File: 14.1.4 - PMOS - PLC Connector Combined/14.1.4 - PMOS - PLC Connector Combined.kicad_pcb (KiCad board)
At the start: 2 copper layers, 61.5 x 67.8 mm, 110 parts, among them J201 Conn_01x01_PAD, J202 Conn_01x01_PAD, J203 Conn_01x01_PAD, J204 Conn_01x01_PAD, J205 Conn_01x01_PAD, J206 Conn_01x01_PAD, J207 Conn_01x01_PAD, J208 Conn_01x01_PAD, J209 Conn_01x01_PAD, J210 Conn_01x01_PAD, J211 Conn_01x01_PAD, J212 Conn_01x01_PAD, J213 Conn_01x01_PAD, J214 Conn_01x01_PAD, J215 Conn_01x01_PAD, J216 Conn_01x01_PAD, J217 Conn_01x01_PAD, J218 Conn_01x01_PAD, J219 Conn_01x01_PAD, J220 Conn_01x01_PAD, J221 DB128L-5.08-2P-BK-S, J222 DB128L-5.08-2P-BK-S, J223 DB128L-5.08-2P-BK-S, J224 DB128L-5.08-2P-BK-S, J225 DB128L-5.08-2P-BK-S, J226 B04B-XASK-1, J301 Conn_01x01_PAD, J302 Conn_01x01_PAD, J303 Conn_01x01_PAD, J304 Conn_01x01_PAD, J305 Conn_01x01_PAD, J306 Conn_01x01_PAD, J307 Conn_01x01_PAD, J308 Conn_01x01_PAD, J309 Conn_01x01_PAD, J310 Conn_01x01_PAD, J311 Conn_01x01_PAD, J312 Conn_01x01_PAD, J313 Conn_01x01_PAD, J314 Conn_01x01_PAD, J315 Conn_01x01_PAD, J316 Conn_01x01_PAD, J317 DB128L-5.08-2P-BK-S, J318 DB128L-5.08-3P-BK-S, J319 DB128L-5.08-2P-BK-S, J320 DB128L-5.08-2P-BK-S, J321 B04B-XASK-1, Q1 2N7002, Q2 2N7002, Q3 2N7002, Q4 2N7002, U1 DMP6023LE-13, U2 DMP6023LE-13, U3 DMP6023LE-13, U4 DMP6023LE-13

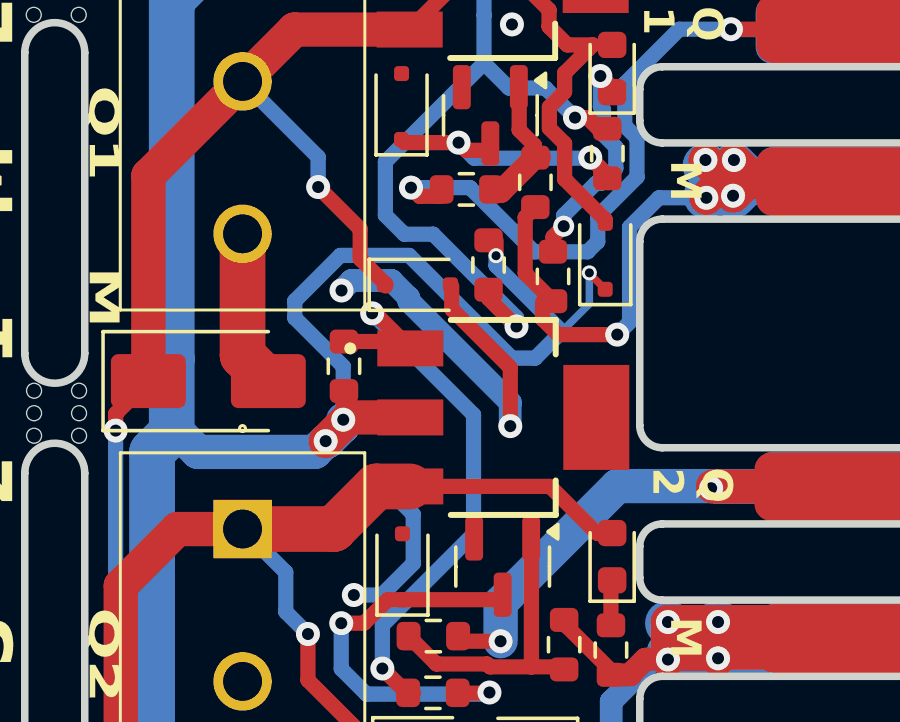
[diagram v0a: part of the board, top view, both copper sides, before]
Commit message: 20241124
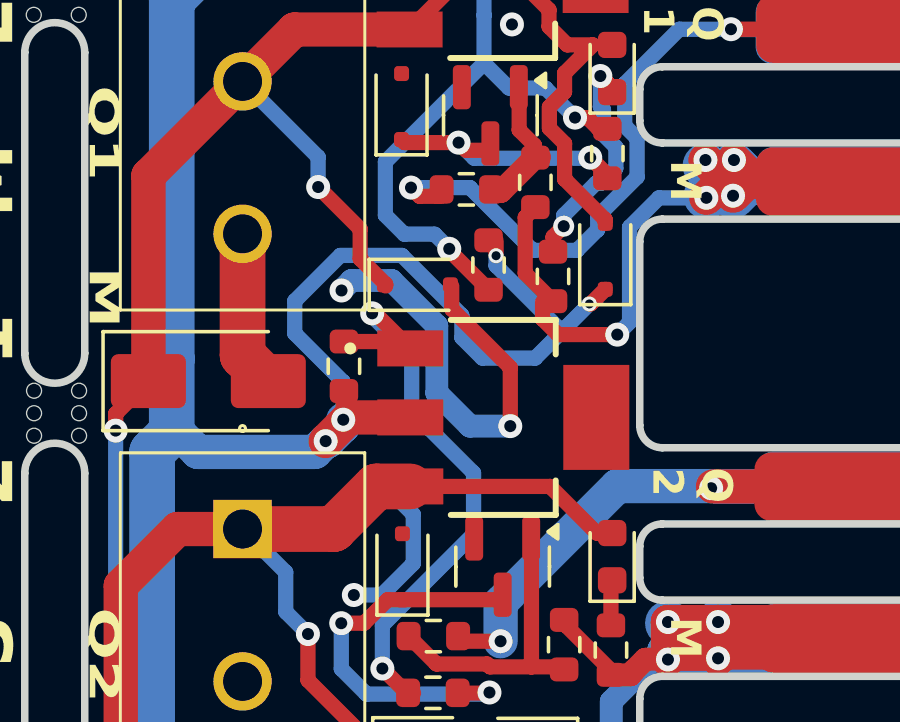
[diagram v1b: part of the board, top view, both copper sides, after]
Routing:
- net Net-(R1-Pad1): track 26.7 -> 23.5 mm
- net GNDPWR: track 278.1 -> 278.9 mm
- net Net-(D10-K): track 142.2 -> 141.6 mm
